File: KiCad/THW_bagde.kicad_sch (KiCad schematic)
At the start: 31 parts, among them J1 USB_B, SW1 SW_Push, SW2 SW_Push, SW3 SW_Push, U1 ATmega32L-8P, Y1 Crystal

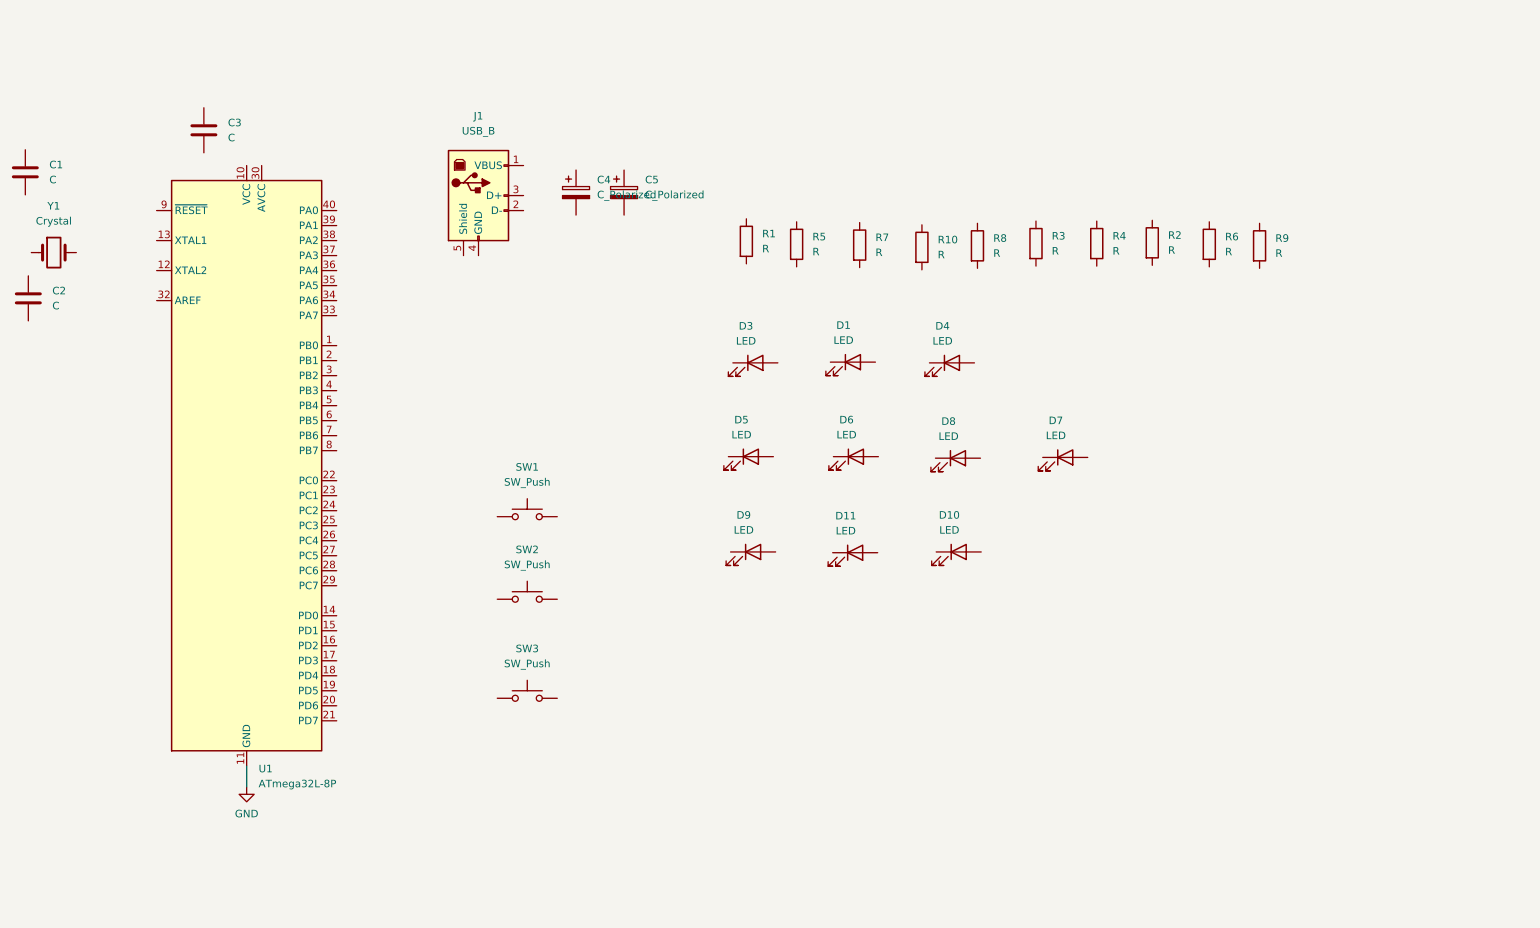
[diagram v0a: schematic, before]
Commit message: adding lugsaar worksheet file
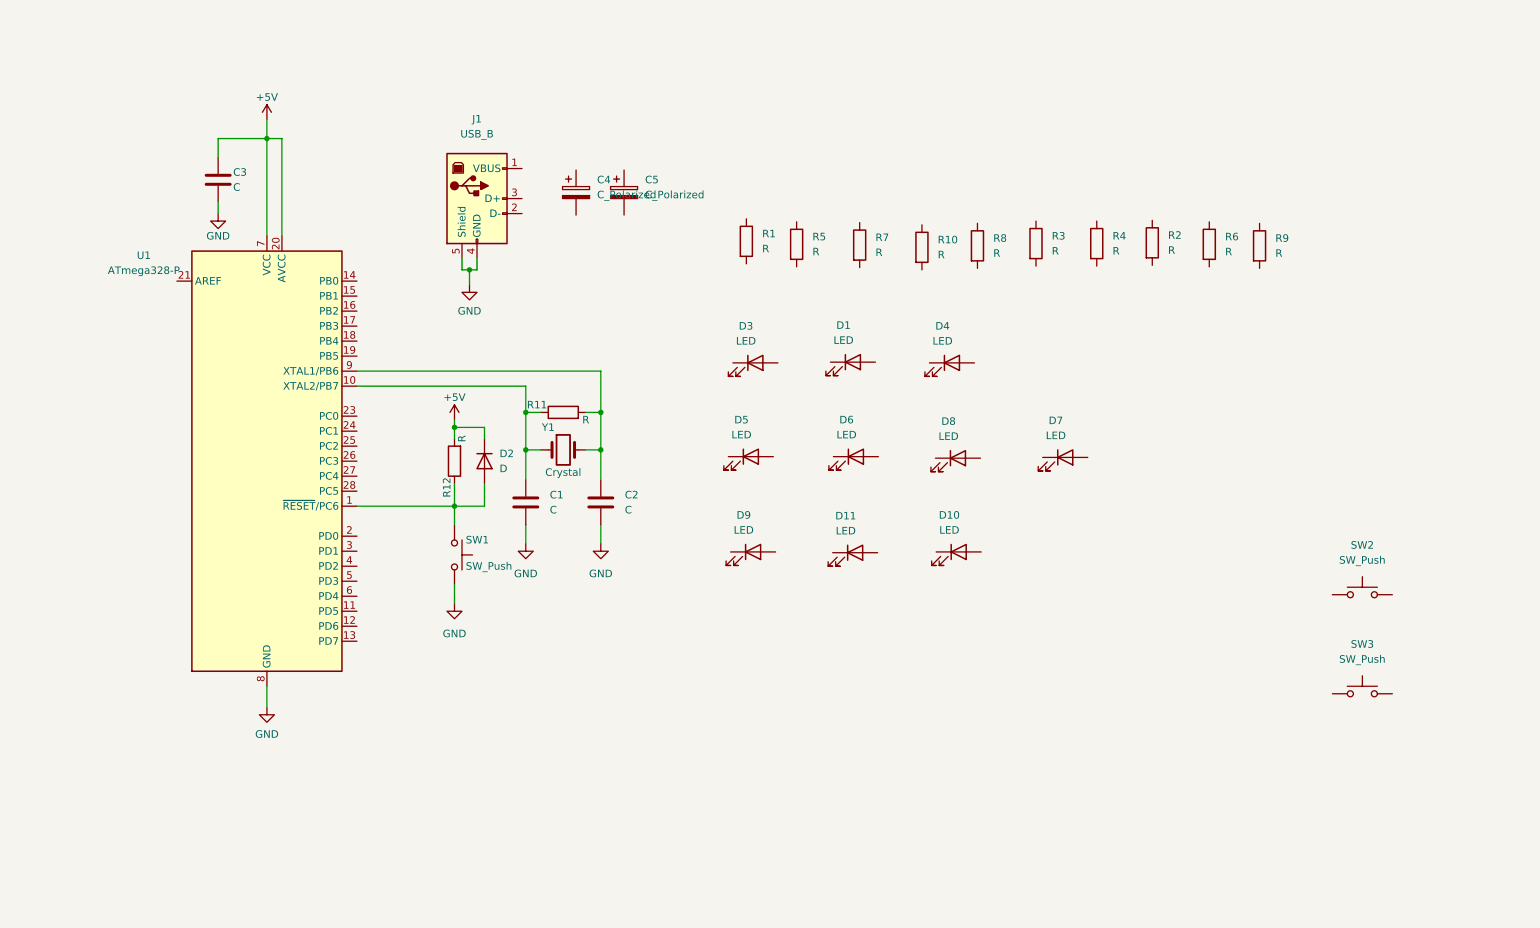
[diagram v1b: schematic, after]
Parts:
- removed U1: ATmega32L-8P, Package_DIP:DIP-40_W15.24mm, symbol MCU_Microchip_ATmega:ATmega32L-8P
- added D2: D, Diode_THT:D_DO-41_SOD81_P10.16mm_Horizontal, symbol Device:D
- added R11, R12: R, Resistor_THT:R_Axial_DIN0207_L6.3mm_D2.5mm_P10.16mm_Horizontal, symbol Device:R
- added U1: ATmega328-P, Package_DIP:DIP-28_W7.62mm, symbol MCU_Microchip_ATmega:ATmega328-P
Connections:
- net GND: now also C1.2, C2.2, C3.2, J1.4 (GND), J1.5 (Shield), SW1.2, U1.22 (GND), U1.8 (GND)
- net at C1.1: now also Y1.1, R11.1, U1.10 (XTAL2/PB7)
- net at C2.1: now also Y1.2, R11.2, U1.9 (XTAL1/PB6)
- net at SW1.1: now also D2.2 (A), R12.1, U1.1 (~{RESET}/PC6)
- net +5V: now reaches C3.1
- net +5V: now also D2.1 (K), R12.2, U1.20 (AVCC), U1.7 (VCC)
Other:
- moved on the sheet: C1, C2, C3, J1, SW1, SW2, SW3, Y1

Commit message: LED placement
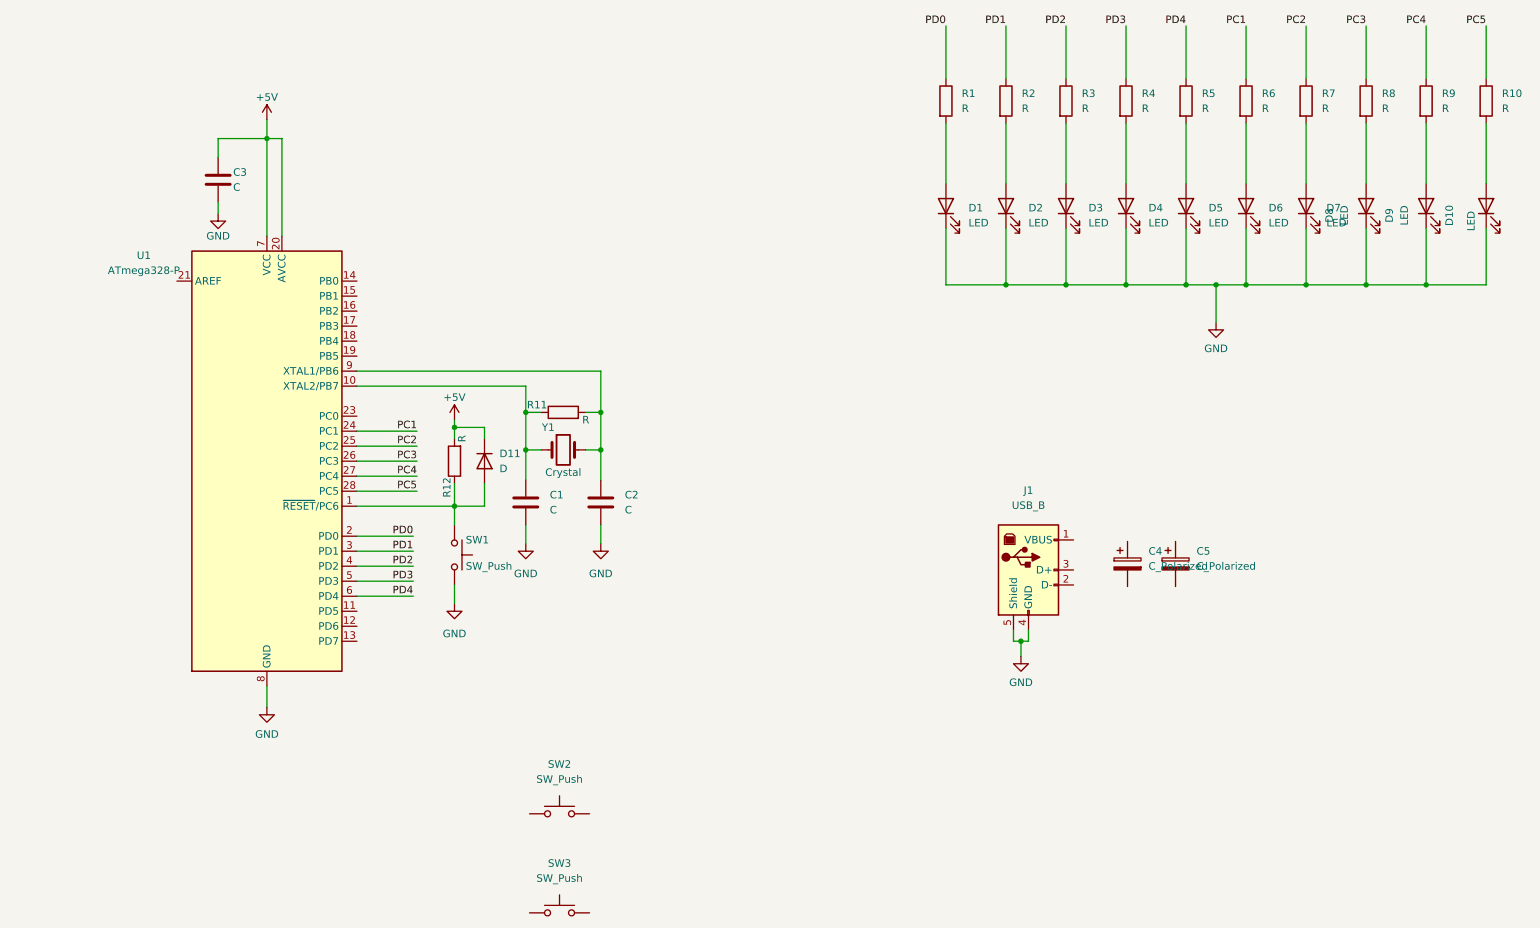
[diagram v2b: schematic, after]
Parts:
- C5: footprint Capacitor_THT:CP_Radial_D10.0mm_P2.50mm -> Capacitor_THT:CP_Radial_D6.3mm_P2.50mm
- renumbered D2 to D11, D11 to D2, R9 to R10, R5 to R2, R7 to R3, R10 to R4, R8 to R5, R3 to R6, R4 to R7, R2 to R8, R6 to R9
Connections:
- net GND: now also D1.1 (K), D10.1 (K), D2.1 (K), D3.1 (K), D4.1 (K), D5.1 (K), D6.1 (K), D7.1 (K), D8.1 (K), D9.1 (K)
- net PC4: now reaches R9.1
- net PC4: now also U1.27 (PC4)
- net at R9.2: now also D9.2 (A)
- net PC3: now reaches R8.1
- net PC3: now also U1.26 (PC3)
- net at R8.2: now also D8.2 (A)
- net PC2: now reaches R7.1
- net PC2: now also U1.25 (PC2)
- net at R7.2: now also D7.2 (A)
- net PD1: now reaches R2.1
- net PD1: now also U1.3 (PD1)
- net at R2.2: now also D2.2 (A)
- net at D1.2 (A): now also R1.2
- net at D3.2 (A): now also R3.2
- net PC1: now reaches R6.1
- net PC1: now also U1.24 (PC1)
- net at R6.2: now also D6.2 (A)
- net PD3: now reaches R4.1
- net PD3: now also U1.5 (PD3)
- net at R4.2: now also D4.2 (A)
- net at D5.2 (A): now also R5.2
- net PD4: now reaches R5.1
- net PD4: now also U1.6 (PD4)
- net PC5: now reaches R10.1
- net PC5: now also U1.28 (PC5)
- net at R10.2: now also D10.2 (A)
- net PD2: now reaches R3.1
- net PD2: now also U1.4 (PD2)
- net PD0: now reaches R1.1
- net PD0: now also U1.2 (PD0)
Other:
- moved on the sheet: C4, C5, D1, D10, D2, D3, D4, D5, D6, D7, D8, D9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
